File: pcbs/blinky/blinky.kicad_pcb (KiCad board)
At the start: 4 copper layers, 135 x 97 mm, 178 parts, among them J1 JACK IN, J3 CA1-9, J4 CB1-9, Q1 PMBT2222A,215, SW1 TACTILE, SW2 JS202011JCQN, U1 ATSAMD21E17, U2 MIC5225-3.3YM5, U3 TSOP36438TT, U4 IS31FL3731-SALS2

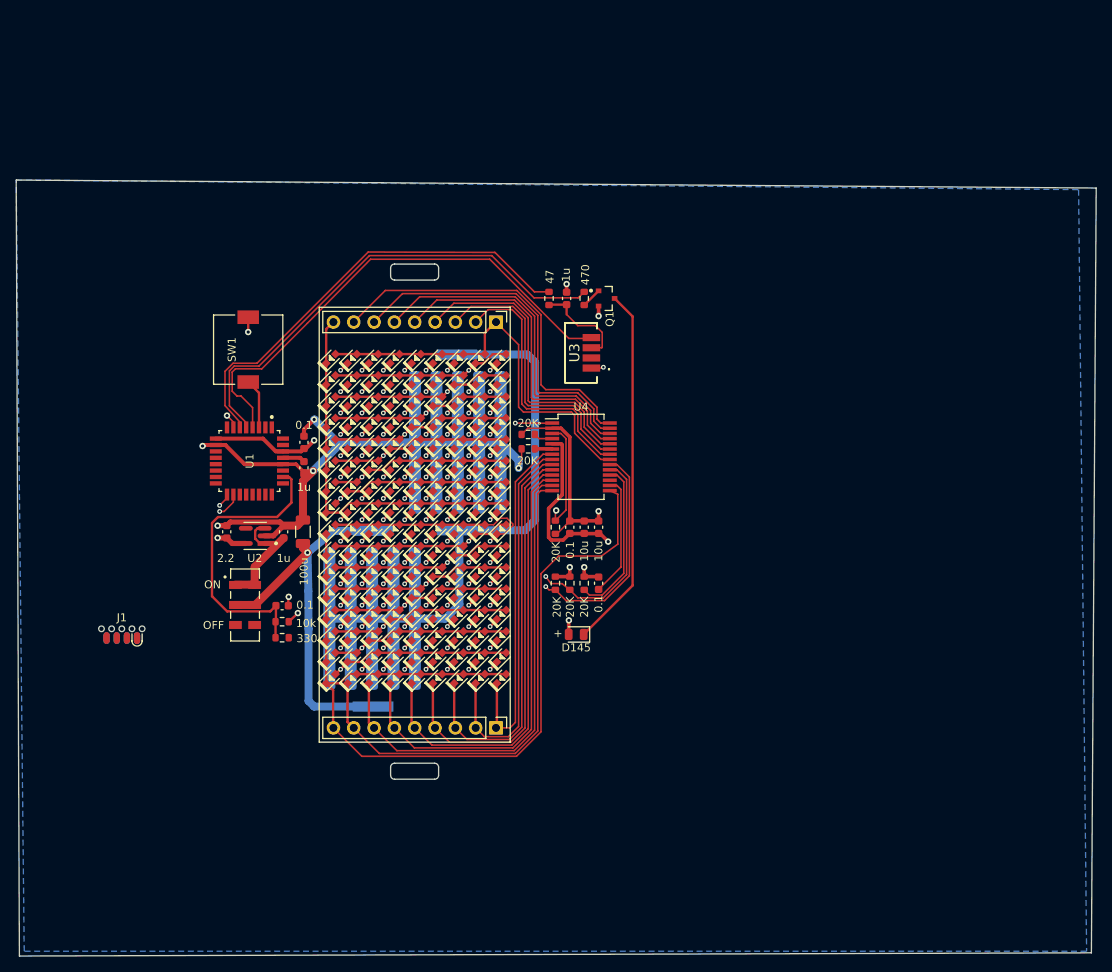
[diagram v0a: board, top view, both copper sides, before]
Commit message: lots of beautiful decorations
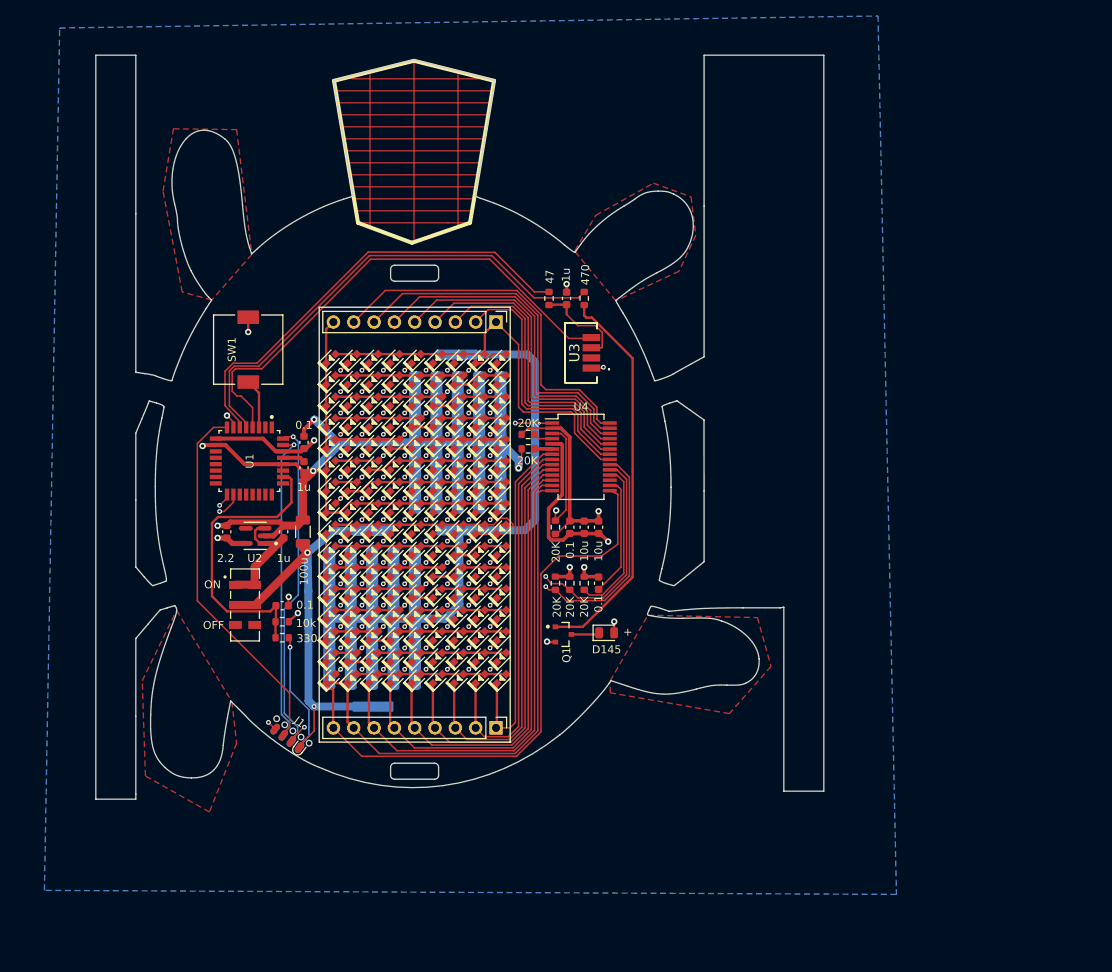
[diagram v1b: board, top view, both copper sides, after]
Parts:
- moved Q1 42.3 mm to (100.7, 141.7)
- moved J1 23.7 mm to (65.7, 155.3), turned to 323 degrees
- moved D145 3.81 mm to (106.1, 141.5), turned to 0 degrees
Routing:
- net (no net): track 0.00 -> 270.2 mm
- net Net-(Q1-Pad1): track 2.54 -> 49.2 mm
- net /A7: track 0.00 -> 46.1 mm
- net Net-(D145-Pad1): track 45.5 -> 3.55 mm
- net /SWDIO: track 0.00 -> 41.5 mm, vias 0 -> 1
- net /SWCLK: track 0.00 -> 39.1 mm, vias 0 -> 1
- net /~RESET: track 0.00 -> 15.2 mm, vias 0 -> 1
- net VBUS: track 49.2 -> 55.0 mm, vias 1 -> 2
- net +3V3: track 48.2 -> 50.3 mm, vias 6 -> 7
- net GND: track 110.7 -> 111.7 mm, vias 12 -> 13
- added copper zone on F.Cu, net (none)
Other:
- board size 135 x 97 mm -> 91 x 93 mm
